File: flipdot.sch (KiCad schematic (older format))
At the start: 41 parts, among them J1 3V3, J2 5V, J3 24V, J4 EN_PWR, J5 Conn_01x02_Male, J6 Conn_01x02_Male, J7 Conn_02x30_Odd_Even, J8 Conn_01x04, J9 Conn_02x30_Odd_Even, U1 74HC595, U10 ULN2803A, U11 ULN2803A, U12 A2982, U13 A2982, U14 A2982, U15 WeMos_D1_mini, U16 ULN2803A, U17 ULN2803A, U18 74HC245, U2 74HC595, U3 74HC595, U4 74HC595, U5 74HC595, U6 74HC595, U7 74HC595, U8 FPF2702MX, U9 ULN2803A

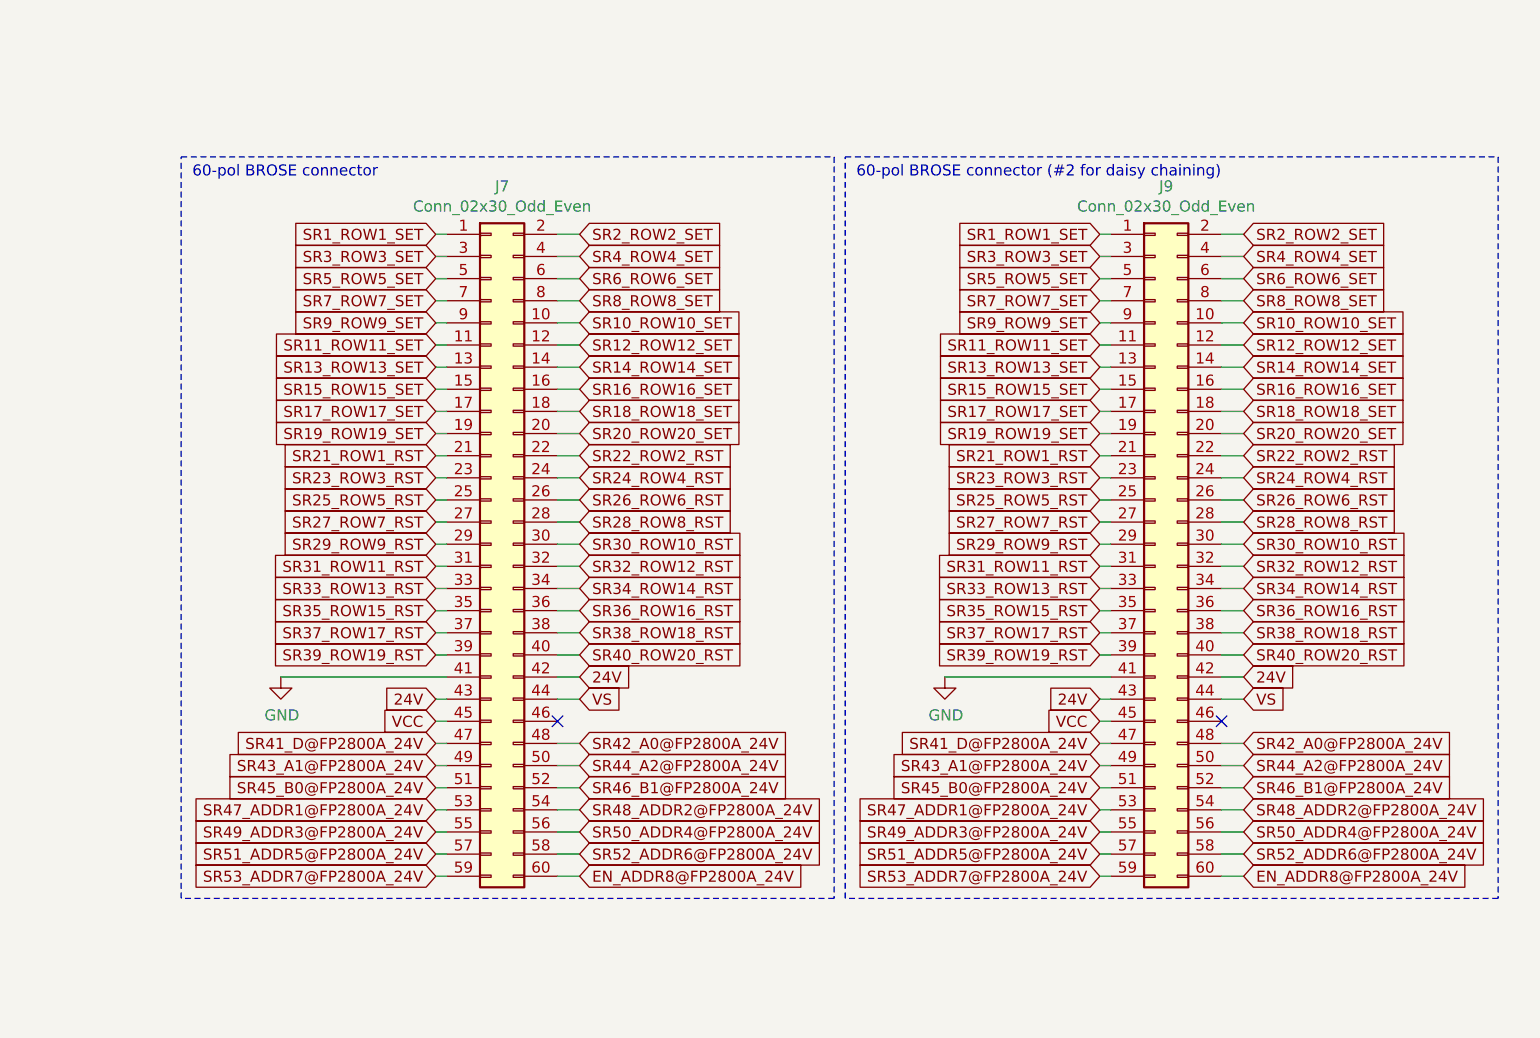
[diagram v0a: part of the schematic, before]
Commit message: update
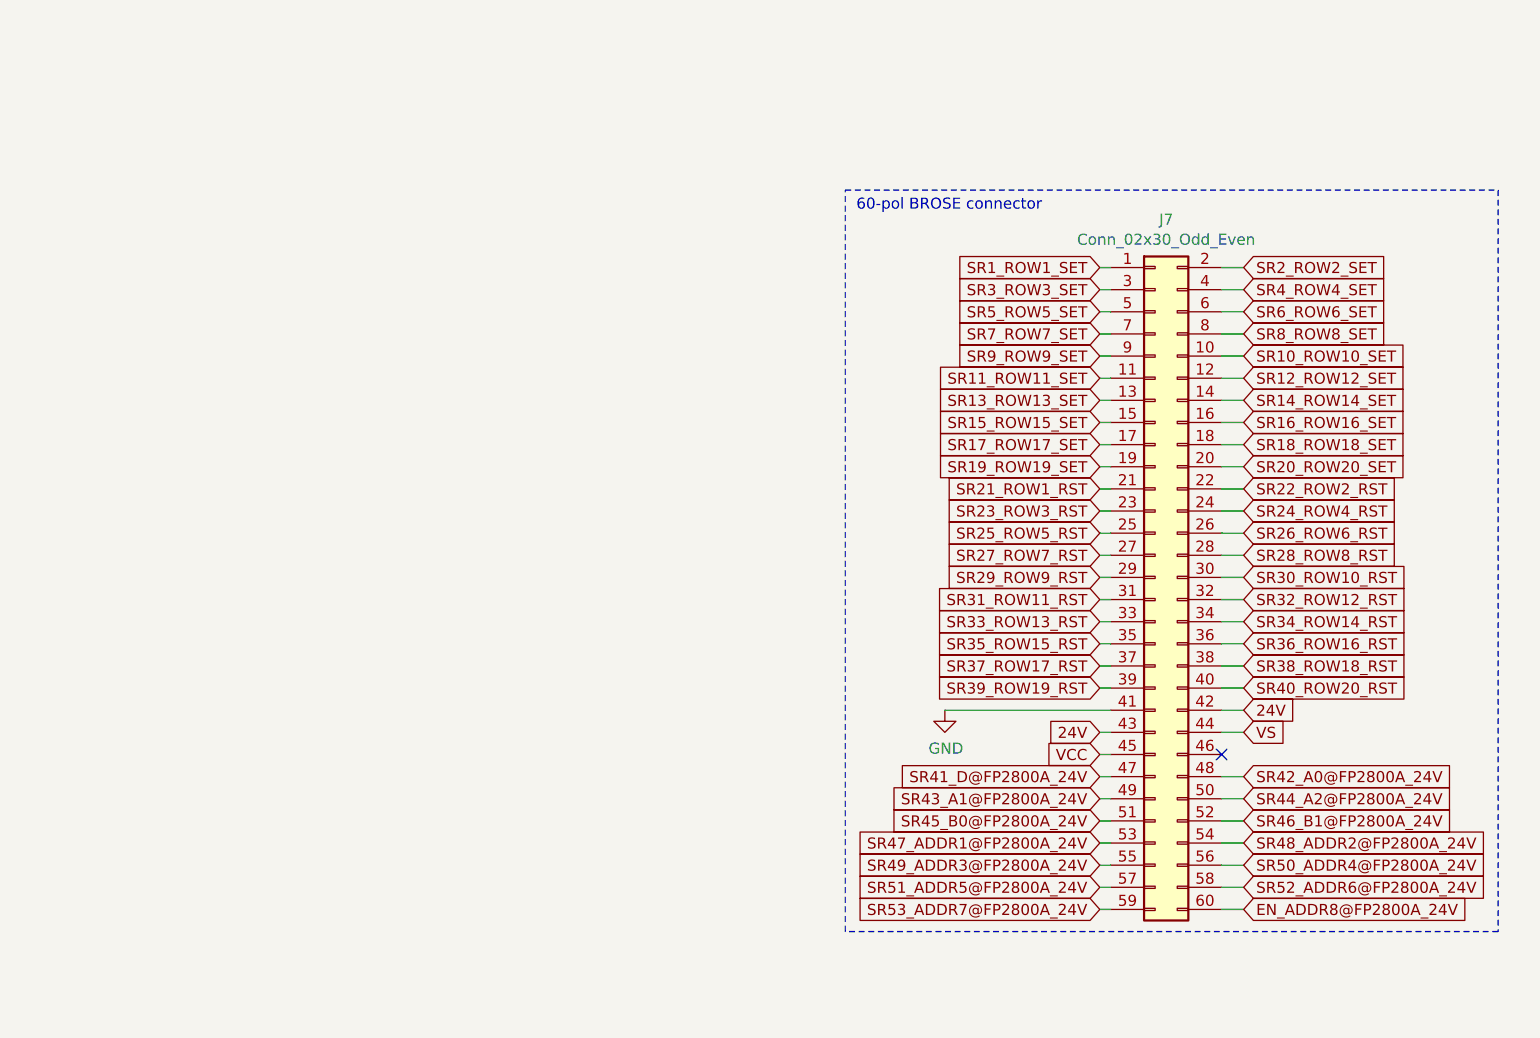
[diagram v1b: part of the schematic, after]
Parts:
- removed J9: Conn_02x30_Odd_Even, Connector_PinHeader_2.54mm:PinHeader_2x30_P2.54mm_Vertical, symbol Connector_Generic:Conn_02x30_Odd_Even
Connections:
- no-connect marks 23 -> 22
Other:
- note removed: "60-pol BROSE connector (#2 for daisy chaining)"
- moved on the sheet: J7
